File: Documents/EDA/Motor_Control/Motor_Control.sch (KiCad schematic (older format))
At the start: 14 parts, among them J1 Power Molex, J2 Barrel_Jack, J3 Pipette, J4 R Home, J5 Z Home, M1 R, M2 Z, U1 ESP32-DEVKITC-32D

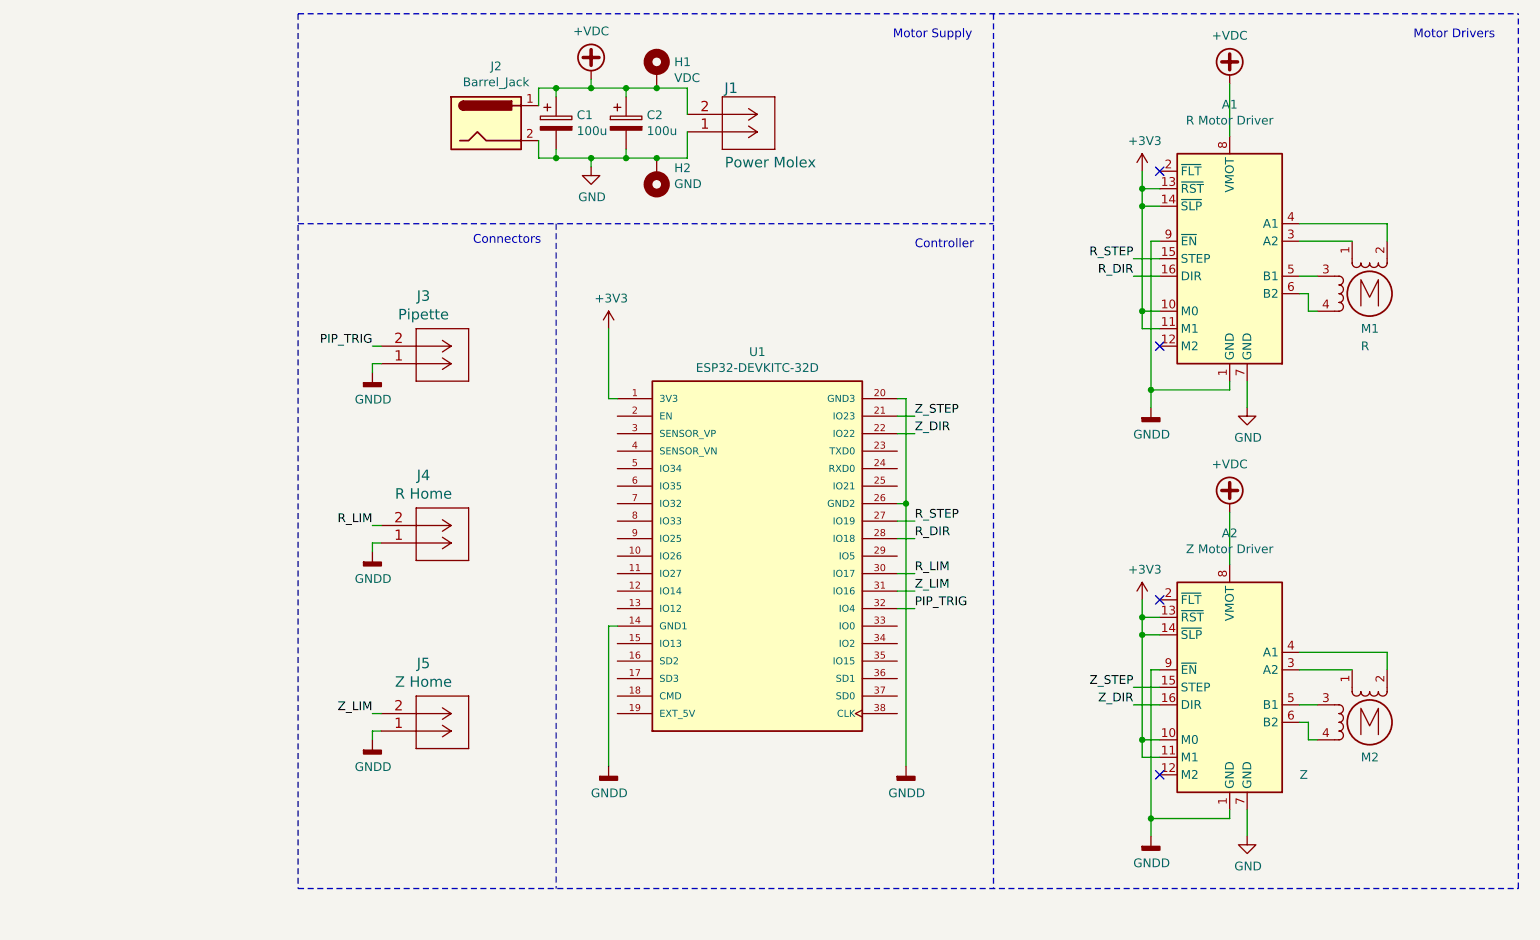
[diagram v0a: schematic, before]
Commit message: Final pcb and bom
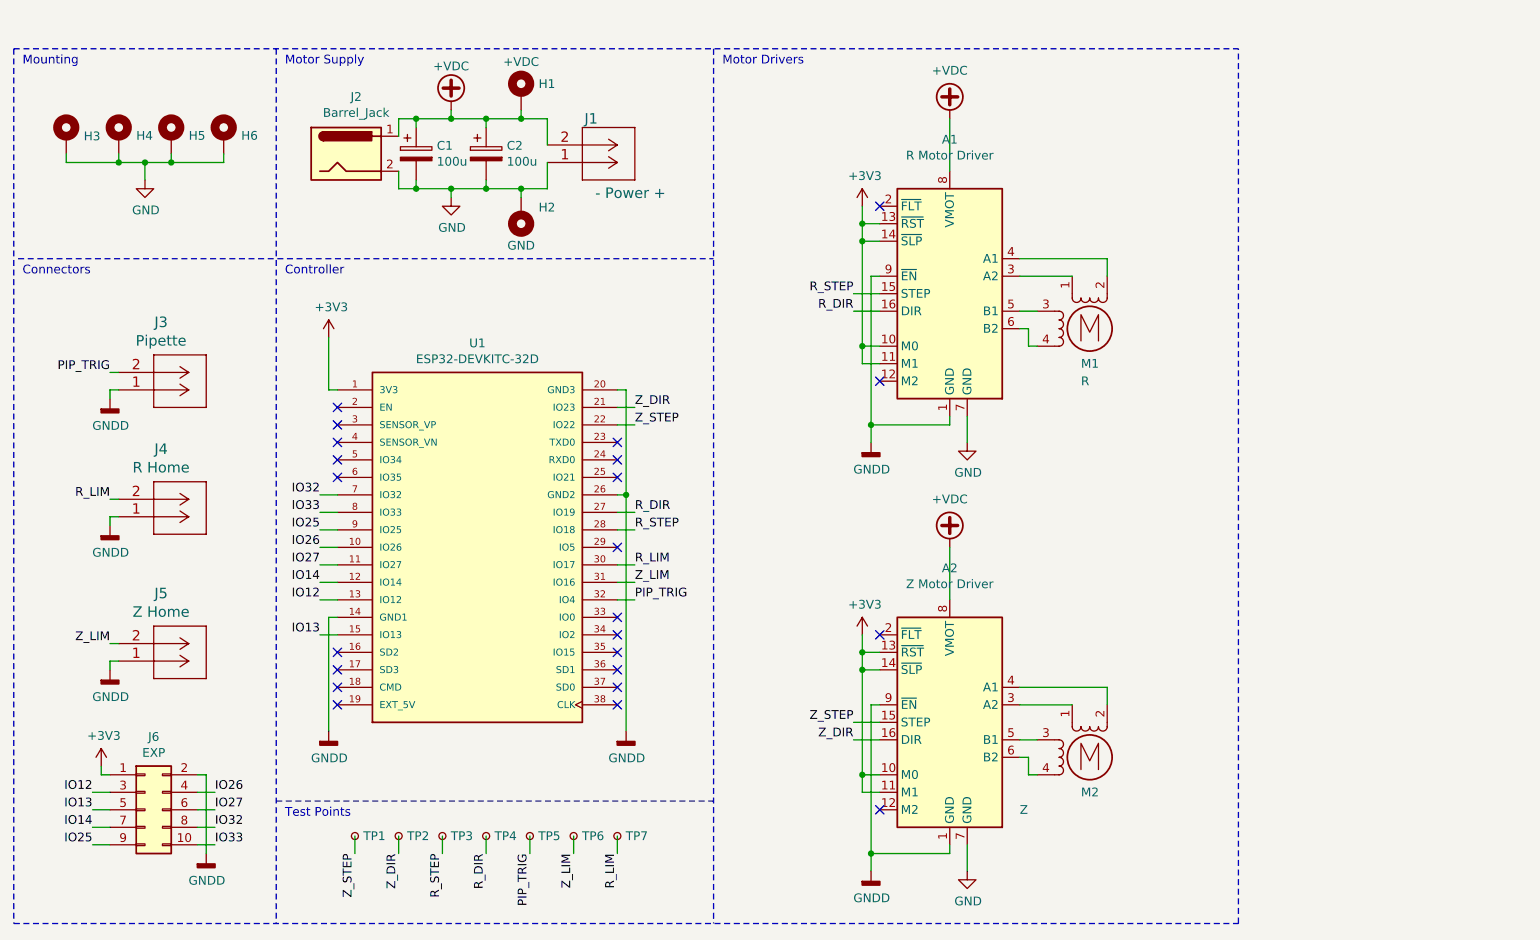
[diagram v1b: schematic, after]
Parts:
- added H3, H4, H5, H6: øM3, MountingHole:MountingHole_3.2mm_M3_Pad_Via, symbol Mechanical:MountingHole_Pad
- added J6: EXP, Connector_PinHeader_2.54mm:PinHeader_2x05_P2.54mm_Vertical, symbol Connector_Generic:Conn_02x05_Odd_Even
- added TP1: Z_STEP, TestPoint:TestPoint_Pad_D1.0mm, symbol Connector:TestPoint_Small
- added TP2: Z_DIR, TestPoint:TestPoint_Pad_D1.0mm, symbol Connector:TestPoint_Small
- added TP3: R_STEP, TestPoint:TestPoint_Pad_D1.0mm, symbol Connector:TestPoint_Small
- added TP4: R_DIR, TestPoint:TestPoint_Pad_D1.0mm, symbol Connector:TestPoint_Small
- added TP5: PIP_TRIG, TestPoint:TestPoint_Pad_D1.0mm, symbol Connector:TestPoint_Small
- added TP6: Z_LIM, TestPoint:TestPoint_Pad_D1.0mm, symbol Connector:TestPoint_Small
- added TP7: R_LIM, TestPoint:TestPoint_Pad_D1.0mm, symbol Connector:TestPoint_Small
- H1: value VDC -> +VDC; footprint MountingHole:MountingHole_3.2mm_M3_Pad_Via -> MountingHole:MountingHole_3.7mm_Pad_Via
- H2: footprint MountingHole:MountingHole_3.2mm_M3_Pad_Via -> MountingHole:MountingHole_3.7mm_Pad_Via
- J1: value Power Molex -> - Power +
- J2: cost (none) -> 1.18; link (none) -> https://www.digikey.co.nz/en/products/detail/cui-devices/PJ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; man part # (none) -> PJ-002BH
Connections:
- net +3V3: now also J6.1 (Pin_1)
- net GND: now also H3.1, H4.1, H5.1, H6.1
- net GNDD: now also J6.2 (Pin_2)
- net PIP_TRIG: now also TP5.1
- net R_DIR: now also U1.27 (IO19), TP4.1; no longer U1.28 (IO18)
- net R_LIM: now also TP7.1
- net R_STEP: now also U1.28 (IO18), TP3.1; no longer U1.27 (IO19)
- net Z_DIR: now also U1.21 (IO23), TP2.1; no longer U1.22 (IO22)
- net Z_LIM: now also TP6.1
- net Z_STEP: now also U1.22 (IO22), TP1.1; no longer U1.21 (IO23)
- net IO26: now reaches U1.10 (IO26)
- net IO26: now also J6.4 (Pin_4)
- net IO27: now reaches U1.11 (IO27)
- net IO27: now also J6.6 (Pin_6)
- net IO14: now reaches U1.12 (IO14)
- net IO14: now also J6.7 (Pin_7)
- net IO12: now reaches U1.13 (IO12)
- net IO12: now also J6.3 (Pin_3)
- net IO13: now reaches U1.15 (IO13)
- net IO13: now also J6.5 (Pin_5)
- net IO32: now reaches U1.7 (IO32)
- net IO32: now also J6.8 (Pin_8)
- net IO33: now reaches U1.8 (IO33)
- net IO33: now also J6.10 (Pin_10)
- net IO25: now reaches U1.9 (IO25)
- net IO25: now also J6.9 (Pin_9)
- no-connect marks 4 -> 23
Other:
- note added: "Mounting\n"
- note added: "Test Points\n"
- moved on the sheet: A1, A2, C1, C2, H1, H2, J1, J2, J3, J4, J5, M1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
